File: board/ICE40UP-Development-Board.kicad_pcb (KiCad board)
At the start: 4 copper layers, 41 x 20.3 mm, 61 parts, among them X1 USB4105-GF-A, X2 Conn_01x16, X3 Conn_01x16, X4 Tag-Connect, Y1 48MHz

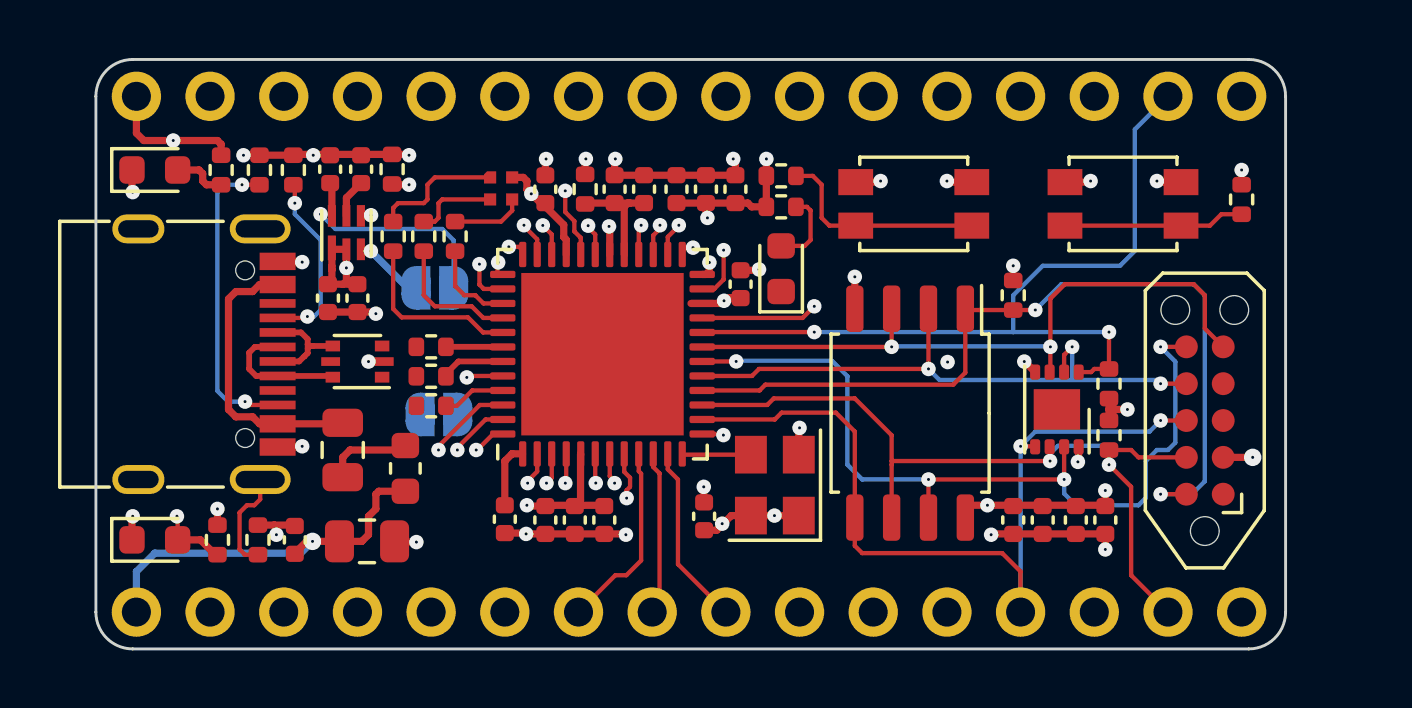
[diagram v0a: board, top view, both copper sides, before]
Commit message: initial pcb layout
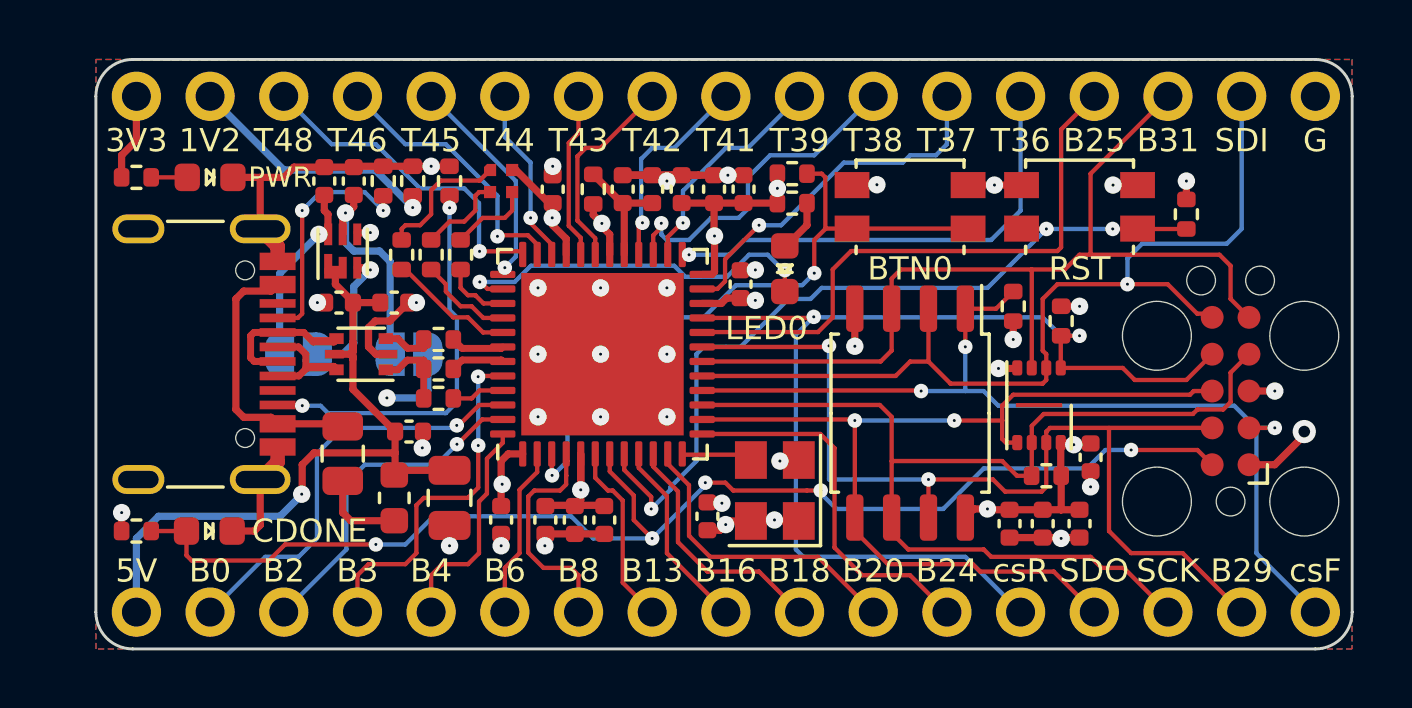
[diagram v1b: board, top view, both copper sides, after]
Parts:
- removed the R6 at (51.3, 94.0)
- X2, X3: value Conn_01x16 -> Conn_01x17; footprint Connector_PinHeader_2.54mm:PinHeader_1x16_P2.54mm_Vertical -> Connector_PinHeader_2.54mm:PinHeader_1x17_P2.54mm_Vertical
- X4: footprint Connector:Tag-Connect_TC2050-IDC-NL_2x05_P1.27mm_Vertical -> Connector:Tag-Connect_TC2050-IDC-FP_2x05_P1.27mm_Vertical
- moved R5 6.56 mm to (57.9, 81.7)
- moved C5 5.43 mm to (56.5, 90.3), turned to 0 degrees
- moved JP1 5.23 mm to (52.7, 87.6), turned to 180 degrees
- moved C3 3.22 mm to (57.9, 92.6), turned to -90 degrees
- moved R4 3.12 mm to (55.6, 81.7)
- moved R16 2.93 mm to (47.1, 81.5), turned to 180 degrees
- moved R17 2.81 mm to (47.1, 93.7), turned to 180 degrees
- moved R3 2.72 mm to (79.0, 86.5), turned to -90 degrees
- moved R1 2.57 mm to (78.5, 91.8), turned to 180 degrees
- moved JP2 2.32 mm to (56.5, 87.6)
- moved C8 2.22 mm to (80.0, 91.2)
- moved R12 1.97 mm to (83.3, 82.8)
- moved V5 1.92 mm to (49.7, 81.5), turned to 180 degrees
- moved V9 1.90 mm to (49.6, 93.7), turned to 180 degrees
- moved S2 1.50 mm to (79.6, 82.5)
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- renumbered C16 to C1, C22 to C10, C13 to C11, C14 to C12, C5 to C13, C6 to C14, C7 to C15, C15 to C16, C8 to C17, C1 to C18, C9 to C19, C17 to C2, C10 to C20, C18 to C21, C2 to C22, C11 to C4, C4 to C5, C12 to C6, C19 to C7, C21 to C8, C20 to C9, R16 to R1, R5 to R10, R15 to R11, R19 to R12, R11 to R13, R12 to R14, R13 to R15, R9 to R16, R18 to R17, R14 to R18, R10 to R2, R17 to R3, R3 to R4, R4 to R5, R8 to R6, R1 to R8, R2 to R9, V5 to V1, V8 to V2, V2 to V4, V4 to V5, V1 to V6, V6 to V7, V7 to V8
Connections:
- C16 pad 1: GND -> +3V3
- C16 pad 2: +3V3 -> GND
- V6 pad 18: SPI_~{HOLD} -> SPI_~{WP}
- V6 pad 19: SPI_~{WP} -> SPI_~{HOLD}
- V6 pad 20: RAM_~{SS} -> IOB_25b
- V6 pad 21: IOB_23b -> RAM_~{SS}
- X1 pad S1: Net-(R6-Pad1) -> GND
- X2 pad 10: IOT_44b -> IOT_39a
- X2 pad 11: IOT_45a -> IOT_38b
- X2 pad 12: IOB_8a -> IOT_37b
- X2 pad 13: IOB_0a -> IOT_36b
- X2 pad 14: IOB_2a -> IOB_25b
- X2 pad 15: RAM_~{SS} -> SPI_~{WP}
- X2 pad 16: GND -> SPI_SI
- X2 pad 3: IOT_36b -> IOT_48b
- X2 pad 4: IOT_37b -> IOT_46b
- X2 pad 5: IOT_38b -> IOT_45a
- X2 pad 6: IOT_39a -> IOT_44b
- X2 pad 7: IOT_41a -> IOT_43a
- X2 pad 9: IOT_43a -> IOT_41a
- X3 pad 10: IOT_46b -> IOB_18a
- X3 pad 11: IOB_23b -> IOB_20a
- X3 pad 13: SPI_SO -> RAM_~{SS}
- X3 pad 14: SPI_SI -> SPI_SO
- X3 pad 16: FLASH_~{SS} -> SPI_~{HOLD}
- X3 pad 2: IOB_3b -> IOB_0a
- X3 pad 3: IOB_4a -> IOB_2a
- X3 pad 4: IOT_48b -> IOB_3b
- X3 pad 5: IOB_6a -> IOB_4a
- X3 pad 6: IOB_13b -> IOB_6a
- X3 pad 7: IOB_16a -> IOB_8a
- X3 pad 8: IOB_18a -> IOB_13b
- X3 pad 9: IOB_20a -> IOB_16a
- X4 pad 1: unconnected-(X4-Pad1) -> +3V3
- X4 pad 10: FLASH_~{SS} -> CDONE
- X4 pad 2: GND -> FLASH_~{SS}
- X4 pad 3: unconnected-(X4-Pad3) -> GND
- X4 pad 4: unconnected-(X4-Pad4) -> SPI_SCK
- X4 pad 6: SPI_~{HOLD} -> SPI_SI
- X4 pad 7: SPI_SI -> RAM_~{SS}
- X4 pad 9: SPI_SCK -> SPI_~{HOLD}
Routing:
- net CDONE: track 3.48 -> 44.3 mm, vias 2 -> 5
- net IOB_25b: track 0.00 -> 20.2 mm
- net ~{RST}: track 8.00 -> 27.8 mm, vias 1 -> 3
- net +1V2: track 9.48 -> 26.0 mm, vias 5 -> 4
- net ~{CONF}_I: track 8.52 -> 24.4 mm, vias 1 -> 2
- net IOT_36b: track 0.56 -> 16.2 mm
- net IOB_24a: track 0.75 -> 13.0 mm, vias 1 -> 0
- net SPI_SI: track 21.2 -> 33.4 mm, vias 3 -> 1
- net IOB_0a: track 2.93 -> 14.8 mm
- net CONF_O: track 1.57 -> 13.1 mm, vias 1 -> 2
- net IOB_3b: track 1.38 -> 12.3 mm, vias 1 -> 2
- net IOT_48b: track 0.67 -> 11.5 mm
- net IOT_37b: track 1.89 -> 12.6 mm
- net IOT_38b: track 1.10 -> 11.6 mm
- net SPI_~{WP}: track 23.6 -> 33.4 mm, vias 2 -> 0
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- added copper zone on B.Cu, net (none)
- added copper zone on F.Cu, net (none)
- added copper zone on In2.Cu, net +1V2
- added copper zone on In2.Cu, net +3V3
- added copper zone on In1.Cu, net GND
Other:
- board size 41 x 20.3 mm -> 43.3 x 20.3 mm
- board text added: "1V2"
- board text added: "3V3"
- board text added: "5V"
- board text added: "B0"
- board text added: "B13"
- board text added: "B16"
- board text added: "B18"
- board text added: "B2"
- board text added: "B20"
- board text added: "B24"
- board text added: "B25"
- board text added: "B29"
- board text added: "B3"
- board text added: "B31"
- board text added: "B4"
- board text added: "B6"
- board text added: "B8"
- board text added: "BTN0"
- board text added: "CDONE"
- board text added: "G"
- board text added: "LED0"
- board text added: "PWR"
- board text added: "RST"
- board text added: "SCK"
- board text added: "SDI"
- board text added: "SDO"
- board text added: "T36"
- board text added: "T37"
- board text added: "T38"
- board text added: "T39"
- board text added: "T41"
- board text added: "T42"
- board text added: "T43"
- board text added: "T44"
- board text added: "T45"
- board text added: "T46"
- board text added: "T48"
- board text added: "csF"
- board text added: "csR"
